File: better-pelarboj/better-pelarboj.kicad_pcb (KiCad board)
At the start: 2 copper layers, 39.2 x 58.3 mm, 55 parts, among them J1 Conn_01x03_Pin, J2 Conn_01x04, J3 Conn_02x01, Q1 AO3400A, Q2 AO3400A, Q3 AO3401A, Q4 AO3400A, SW1 SW_Push, SW2 SW_SPST, U1 XIAO-ESP32-C3-DIP, U2 TP5100_C379389, U3 MT3608, U5 AP63205WU

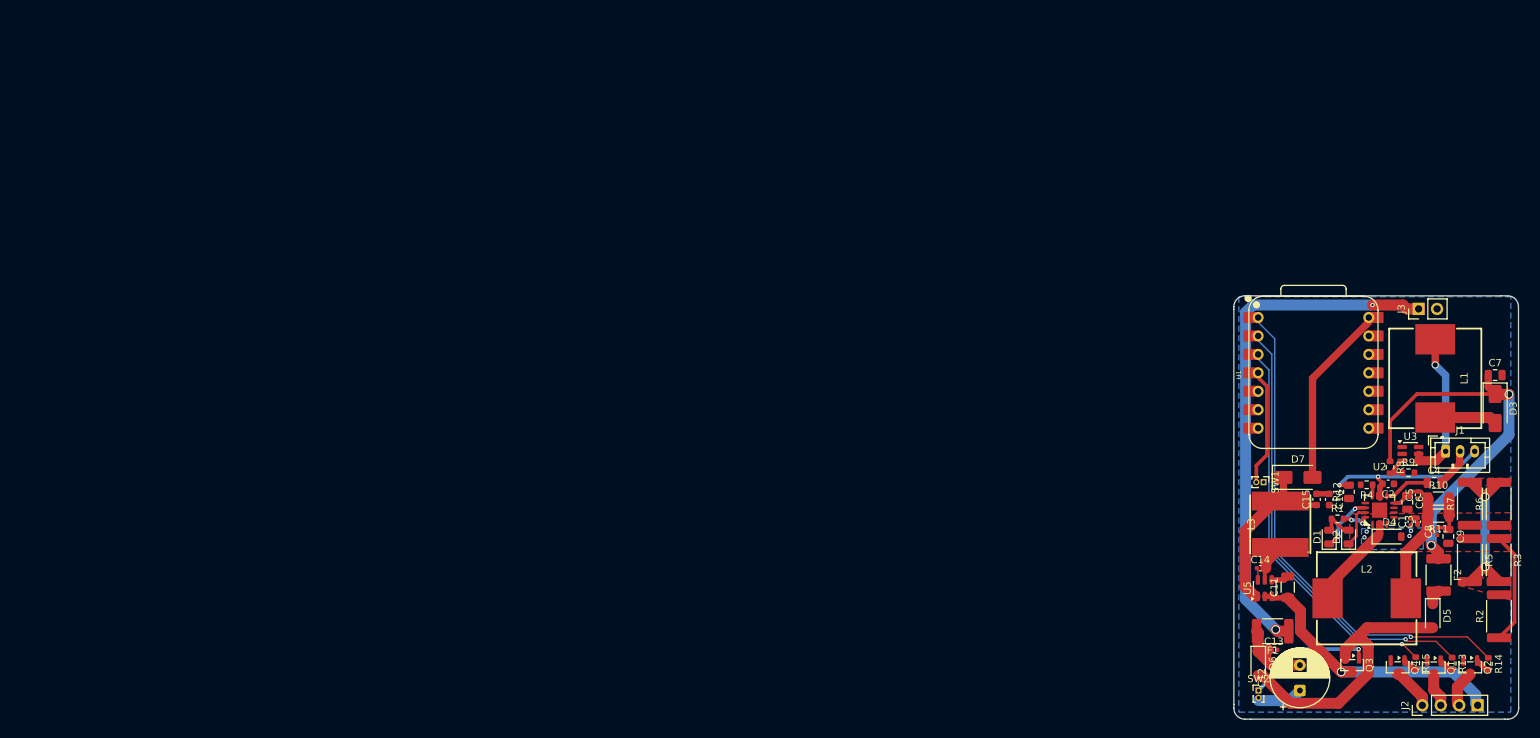
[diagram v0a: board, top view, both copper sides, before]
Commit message: pcb done agaiin (fixed lots of drc and designators. ooh, also a cool 90 deg button
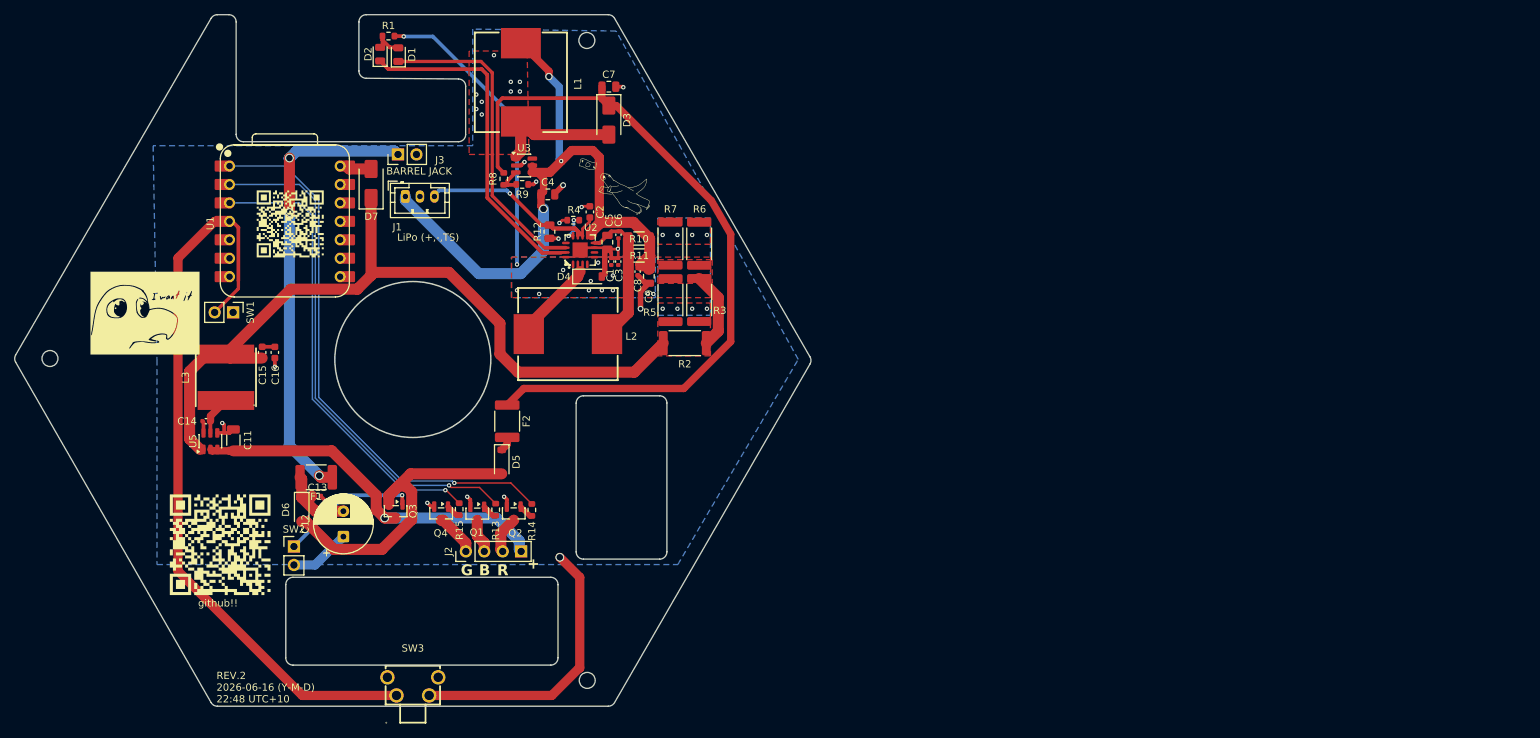
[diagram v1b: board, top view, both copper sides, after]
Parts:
- added G***: LOGO, LOGO, F.Cu at (70.6, 83.8)
- added G***: LOGO, LOGO, F.Cu at (115.3, 79.2)
- added G***: LOGO, LOGO, F.Cu at (50.6, 96.1)
- added G***: LOGO, LOGO, F.Cu at (61.0, 128.0)
- added G***: LOGO, LOGO, B.Cu at (55.1, 105.5)
- added G***: LOGO, LOGO, B.Cu at (87.9, 122.9)
- added H1: MountingHole, MountingHole:MountingHole_2.2mm_M2, F.Cu at (37.5, 102.4)
- added H2: MountingHole, MountingHole:MountingHole_2.2mm_M2, F.Cu at (111.5, 58.6)
- added H3: MountingHole, MountingHole:MountingHole_2.2mm_M2, F.Cu at (111.5, 146.7)
- added SW3: SW_Push, easyeda2kicad:SW-TH_TS665ZJ, F.Cu at (87.5, 147.5)
- SW1, SW2: footprint Connector_PinHeader_1.00mm:PinHeader_1x02_P1.00mm_Vertical -> Connector_PinHeader_2.54mm:PinHeader_1x02_P2.54mm_Vertical
- moved D2 149.1 mm to (83.0, 60.4)
- moved J1 147.5 mm to (86.5, 80.0)
- moved R1 146.7 mm to (84.1, 57.9)
- moved C11 146.7 mm to (62.8, 113.6)
- moved C14 146.7 mm to (59.0, 111.0)
- moved C15 146.7 mm to (66.8, 101.5)
- moved C16 146.7 mm to (68.5, 101.5)
- moved L3 146.7 mm to (61.8, 105.0)
- moved U5 146.7 mm to (59.6, 113.8)
- moved D1 144.4 mm to (85.5, 60.5)
- moved SW1 143.9 mm to (62.7, 96.0)
- moved U1 143.2 mm to (69.9, 83.5)
- moved J3 142.2 mm to (85.5, 74.2)
- moved SW2 134.4 mm to (71.1, 128.3)
- moved D7 134.0 mm to (81.8, 78.2), turned to 90 degrees
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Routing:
- net Net-(U1-GPIO5_A3_D3): track 15.5 -> 104.1 mm
- net GND: track 14.1 -> 87.2 mm, vias 0 -> 25
- net LiPO+: track 33.4 -> 93.1 mm, vias 1 -> 3
- net +5V: track 49.5 -> 108.0 mm, vias 2 -> 8
- net /LiPo_24v: track 54.0 -> 101.8 mm, vias 2 -> 0
- net Net-(D2-K): track 5.80 -> 46.5 mm
- net Net-(D1-K): track 7.92 -> 43.6 mm, vias 2 -> 0
- net Net-(C1-Pad1): track 20.2 -> 52.2 mm, vias 2 -> 13
- net Net-(D7-A): track 24.6 -> 3.59 mm
- net +24V: track 39.4 -> 52.2 mm
- net BLUE_X: track 60.8 -> 70.8 mm
- net GREEN_X: track 53.5 -> 63.6 mm
- net Net-(D3-A): track 8.57 -> 18.0 mm
- net RED_X: track 68.0 -> 76.9 mm
- net Net-(J3-Pin_1): track 71.7 -> 62.9 mm, vias 2 -> 3
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- added copper zone on B.Cu, net +5V
- added copper zone on F.Cu, net GND
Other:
- board size 39.2 x 58.3 mm -> 109.7 x 95.3 mm
- board text added: "+"
- board text added: "- LiPo temperature protection cutoff - Fits seemlessly under the LED module"
- board text added: "A mod for the Ikea Pencil Light, created by @obob Features - XIAO ESP32-3C - Can use both LiPo AND Barrel Jack - Can charge LiPo when on mains (4000mAh at 0.5C)"
- board text added: "B"
- board text added: "BARREL JACK"
- board text added: "Flytboj"
- board text added: "G"
- board text added: "LiPo (+,-,TS)"
- board text added: "R"
- board text added: "REV.2 2026-06-16 (Y-M-D) 22:48 UTC+10"
- board text added: "barrel jack should be facing ^^ too"
- board text added: "flytboj means floating buoy in swedish, {dblquote}floating{dblquote} above the pelarboj void!"
- board text added: "github!!"
